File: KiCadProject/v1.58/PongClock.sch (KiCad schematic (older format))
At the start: 26 parts, among them J1 CONN_01X01_MALE, J2 MY_USB_OTG, SW1 SW_DIP_x01, SW2 SW_DIP_x01, U1 TinyRTC_I2C_RIGHT, U2 MAX7219_IN, U3 MAX7219_IN, U4 MAX7219_IN, U5 MAX7219_IN, U6 MAX7219_IN, U7 MAX7219_IN, U8 ATMEGA328P-PU, U9 FTDI1232, Y1 Crystal

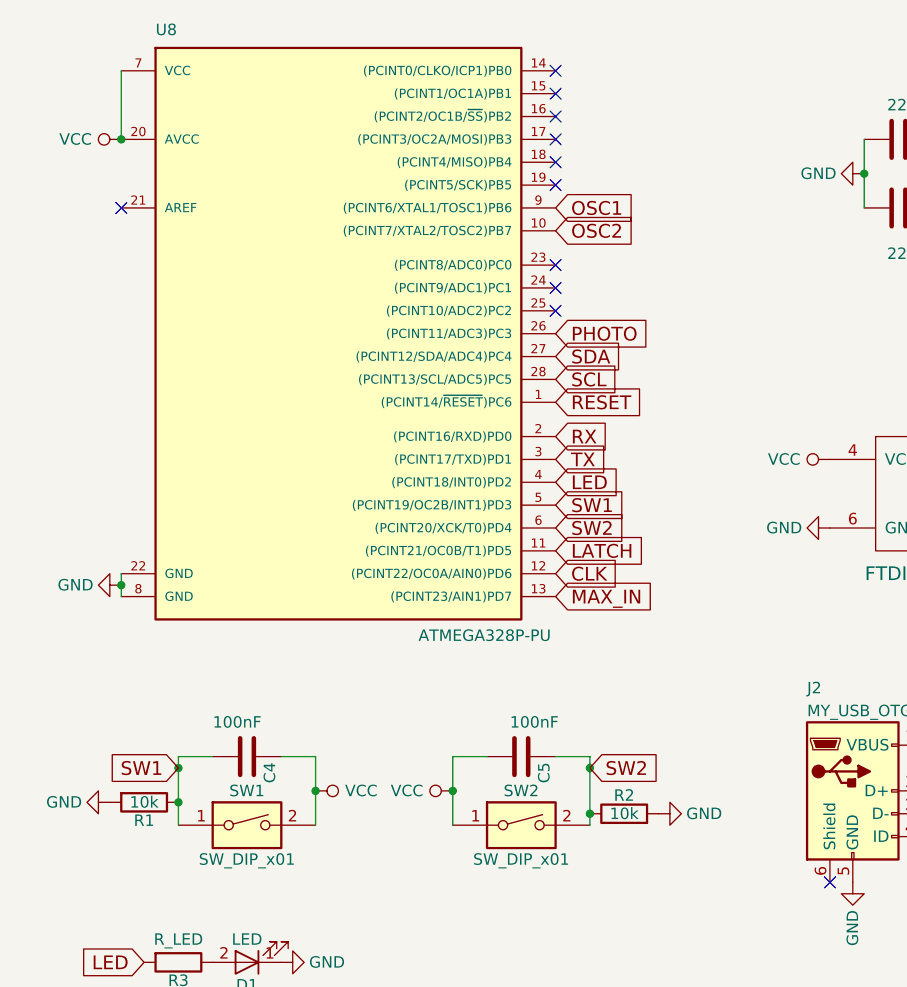
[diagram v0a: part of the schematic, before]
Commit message: v1.58
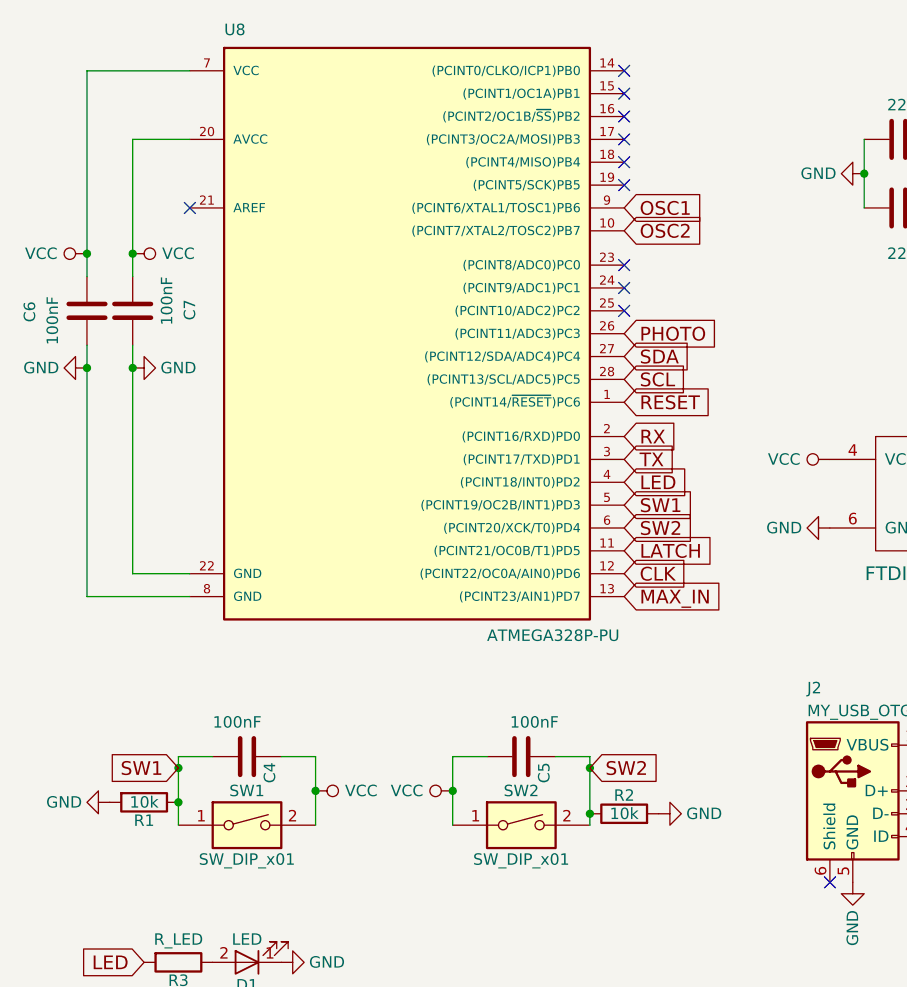
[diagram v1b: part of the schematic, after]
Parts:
- added C6, C7: 100nF, Capacitors_SMD:C_1206_HandSoldering, symbol C
- C1, C2: footprint Capacitors_THT:C_Disc_D3.0mm_W1.6mm_P2.50mm -> Capacitors_SMD:C_1206_HandSoldering
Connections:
- net GND: now also C6.2, C7.1
- net VCC: now also C6.1, C7.2
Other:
- moved on the sheet: U8
